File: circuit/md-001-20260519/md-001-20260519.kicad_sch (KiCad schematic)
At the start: 38 parts, among them J1 VIN-motor, J2 Conn-relay

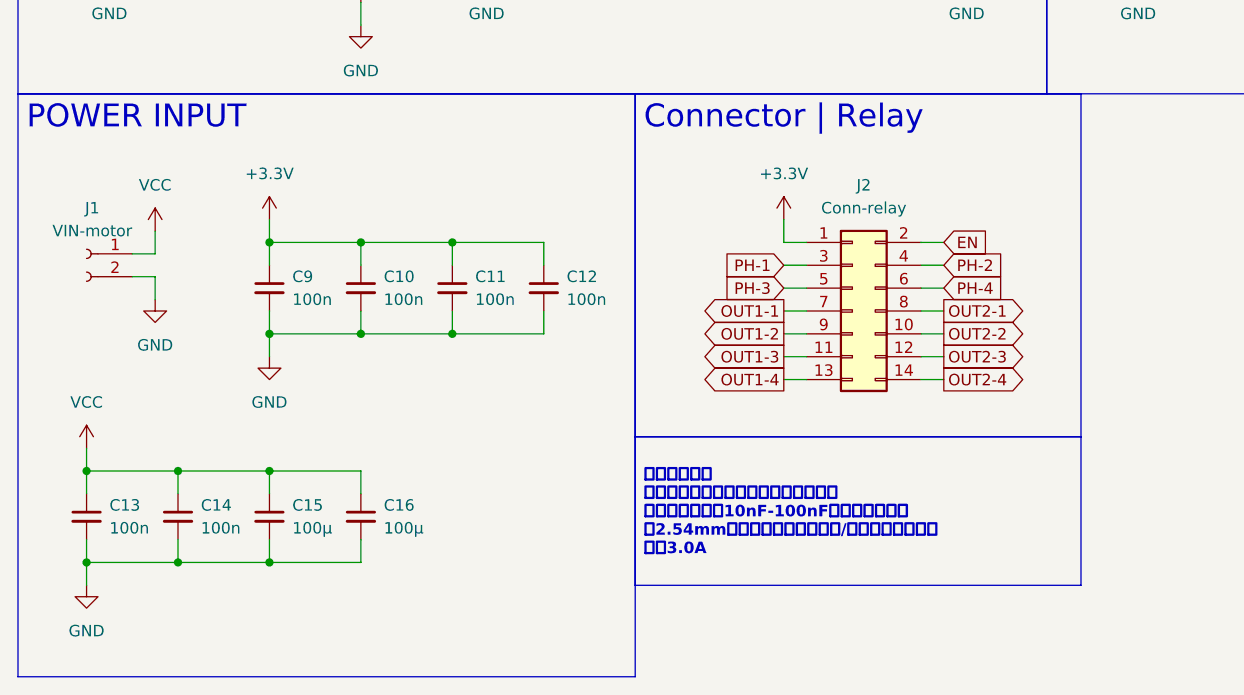
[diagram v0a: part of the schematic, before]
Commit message: Update いったんMD完成
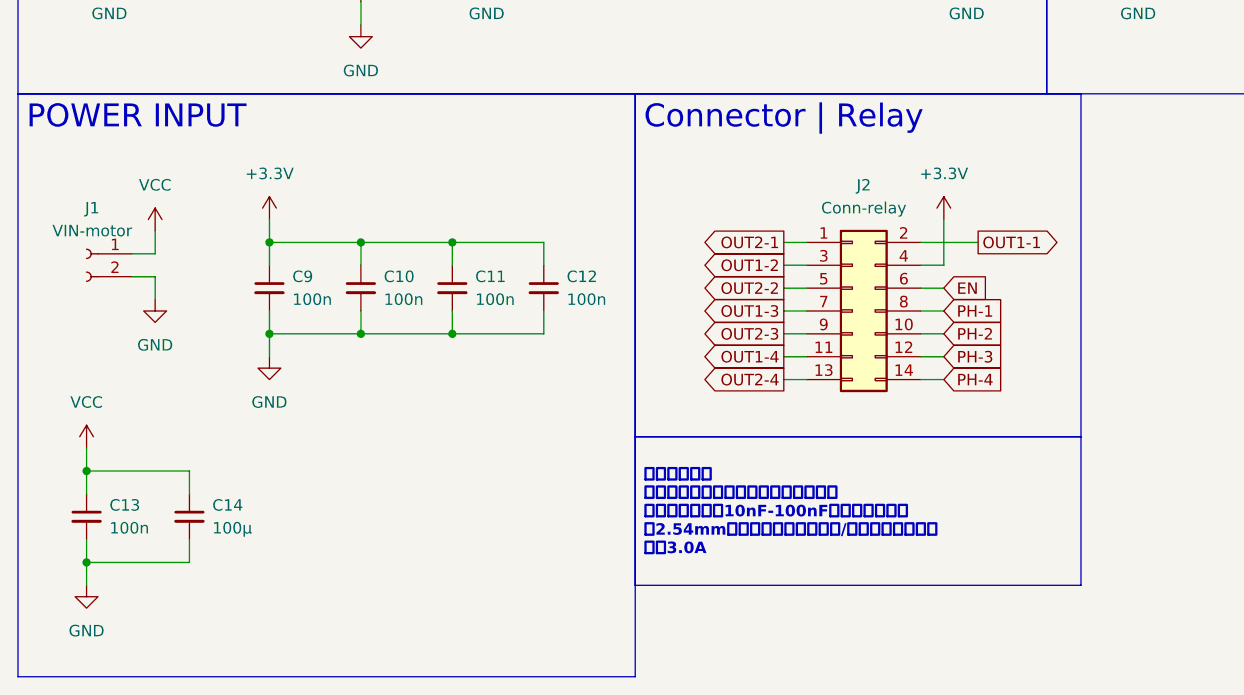
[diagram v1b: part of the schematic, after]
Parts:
- removed C14: 100n, Resistor_SMD:R_0603_1608Metric, symbol Device:C_Small
- removed C16: 100μ, Resistor_SMD:R_1206_3216Metric, symbol Device:C_Small
- renumbered C15 to C14
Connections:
- net +3.3V: now also J2.4 (Pin_4); no longer J2.1 (Pin_1)
- net EN: now also J2.6 (Pin_6); no longer J2.2 (Pin_2)
- net OUT1-1: now also J2.2 (Pin_2); no longer J2.7 (Pin_7)
- net OUT1-2: now also J2.3 (Pin_3); no longer J2.9 (Pin_9)
- net OUT1-3: now also J2.7 (Pin_7); no longer J2.11 (Pin_11)
- net OUT1-4: now also J2.11 (Pin_11); no longer J2.13 (Pin_13)
- net OUT2-1: now also J2.1 (Pin_1); no longer J2.8 (Pin_8)
- net OUT2-2: now also J2.5 (Pin_5); no longer J2.10 (Pin_10)
- net OUT2-3: now also J2.9 (Pin_9); no longer J2.12 (Pin_12)
- net OUT2-4: now also J2.13 (Pin_13); no longer J2.14 (Pin_14)
- net PH-1: now also J2.8 (Pin_8); no longer J2.3 (Pin_3)
- net PH-2: now also J2.10 (Pin_10); no longer J2.4 (Pin_4)
- net PH-3: now also J2.12 (Pin_12); no longer J2.5 (Pin_5)
- net PH-4: now also J2.14 (Pin_14); no longer J2.6 (Pin_6)
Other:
- moved on the sheet: C14
